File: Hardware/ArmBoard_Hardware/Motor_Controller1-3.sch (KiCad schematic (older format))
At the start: 9 parts, among them U6 TB67H400AFNG,EL, U7 TB67H400AFNG,EL, U9 TB67H400AFNG,EL

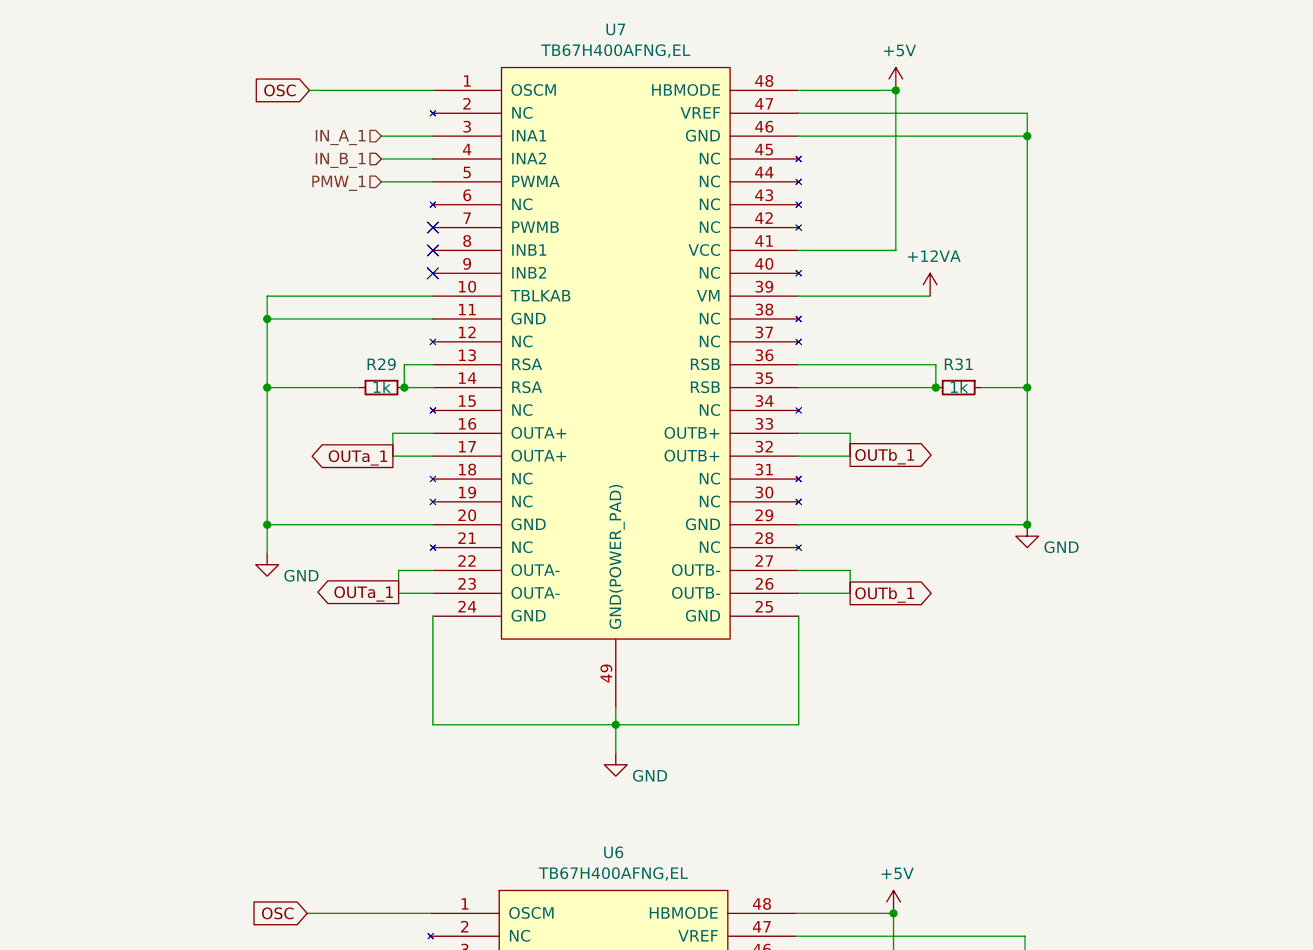
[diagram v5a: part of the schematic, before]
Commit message: rev2 begins
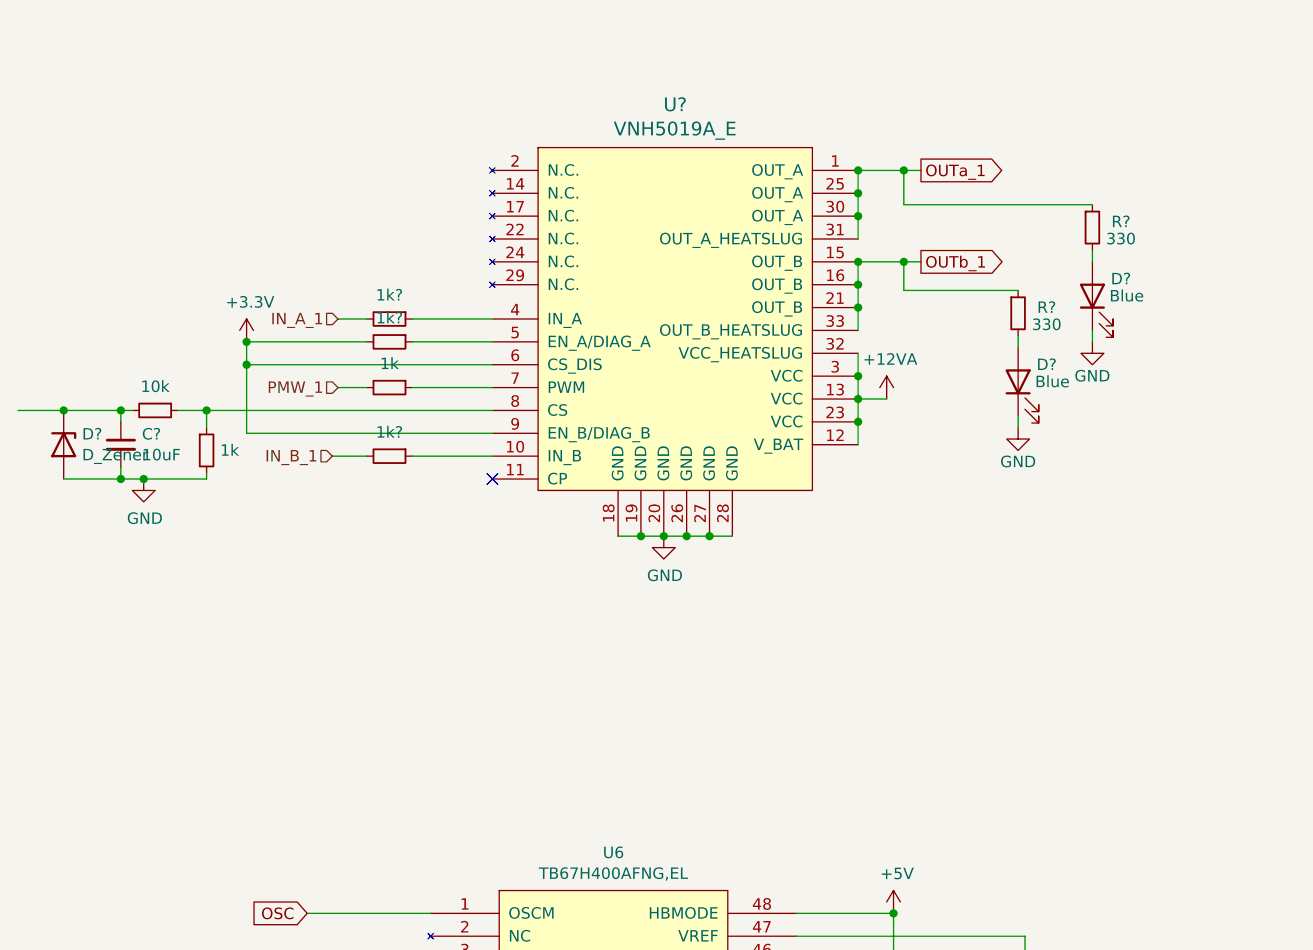
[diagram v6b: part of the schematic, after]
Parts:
- removed R29, R31: 1k, Resistor_SMD:R_0603_1608Metric_Pad0.98x0.95mm_HandSolder, symbol Device:R_Small
- removed U7: TB67H400AFNG,EL, MRDT_ICs:TB67H400AFNG,EL, symbol MRDT_ICs:TB67H400AFNG,EL
- added 10k, 1k (x2), 1k? (x3): R_Small, symbol Device:R_Small
- added C?: 10uF, Capacitor_SMD:C_0603_1608Metric_Pad1.08x0.95mm_HandSolder, symbol Device:C_Small
- added D?: D_Zener, symbol Device:D_Zener
- added D? (x2): Blue, LED_SMD:LED_0603_1608Metric_Pad1.05x0.95mm_HandSolder, symbol Device:LED
- added R? (x2): 330, Resistor_SMD:R_0603_1608Metric_Pad0.98x0.95mm_HandSolder, symbol Device:R_Small
- added U?: VNH5019A_E, symbol MRDT_ICs:VNH5019A_E
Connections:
- net +12VA: now also U?.12 (V_BAT), U?.13 (VCC), U?.23 (VCC), U?.3 (VCC), U?.32 (VCC_HEATSLUG)
- net GND: now also 1k.2, C?.2, D?.1 (K), D?.1 (K), D?.2 (A), U?.18 (GND), U?.19 (GND), U?.20 (GND), U?.26 (GND), U?.27 (GND), U?.28 (GND)
- net IN_A_1: now also 1k?.2
- net IN_B_1: now also 1k?.2
- net OUTa_1: now also R?.1, U?.1 (OUT_A), U?.25 (OUT_A), U?.30 (OUT_A), U?.31 (OUT_A_HEATSLUG)
- net OUTb_1: now also R?.1, U?.15 (OUT_B), U?.16 (OUT_B), U?.21 (OUT_B), U?.33 (OUT_B_HEATSLUG)
- net PMW_1: now also 1k.2
- new net: 1k?.1, U?.10 (IN_B)
- new net: 1k?.1, U?.4 (IN_A)
- new net: 1k?.1, U?.5 (EN_A/DIAG_A)
- new net: 1k.1, U?.7 (PWM)
- new net: 10k.1, 1k.1, U?.8 (CS)
- new net: 10k.2, C?.1, D?.1 (K)
- new net: D?.2 (A), R?.2 (x2)
- new net +3V3: 1k?.2, U?.6 (CS_DIS), U?.9 (EN_B/DIAG_B)
- no-connect marks 9 -> 7
